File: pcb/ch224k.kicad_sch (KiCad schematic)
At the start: 3 parts, among them SW1 SW_Push_DPDT, U2 CH224K

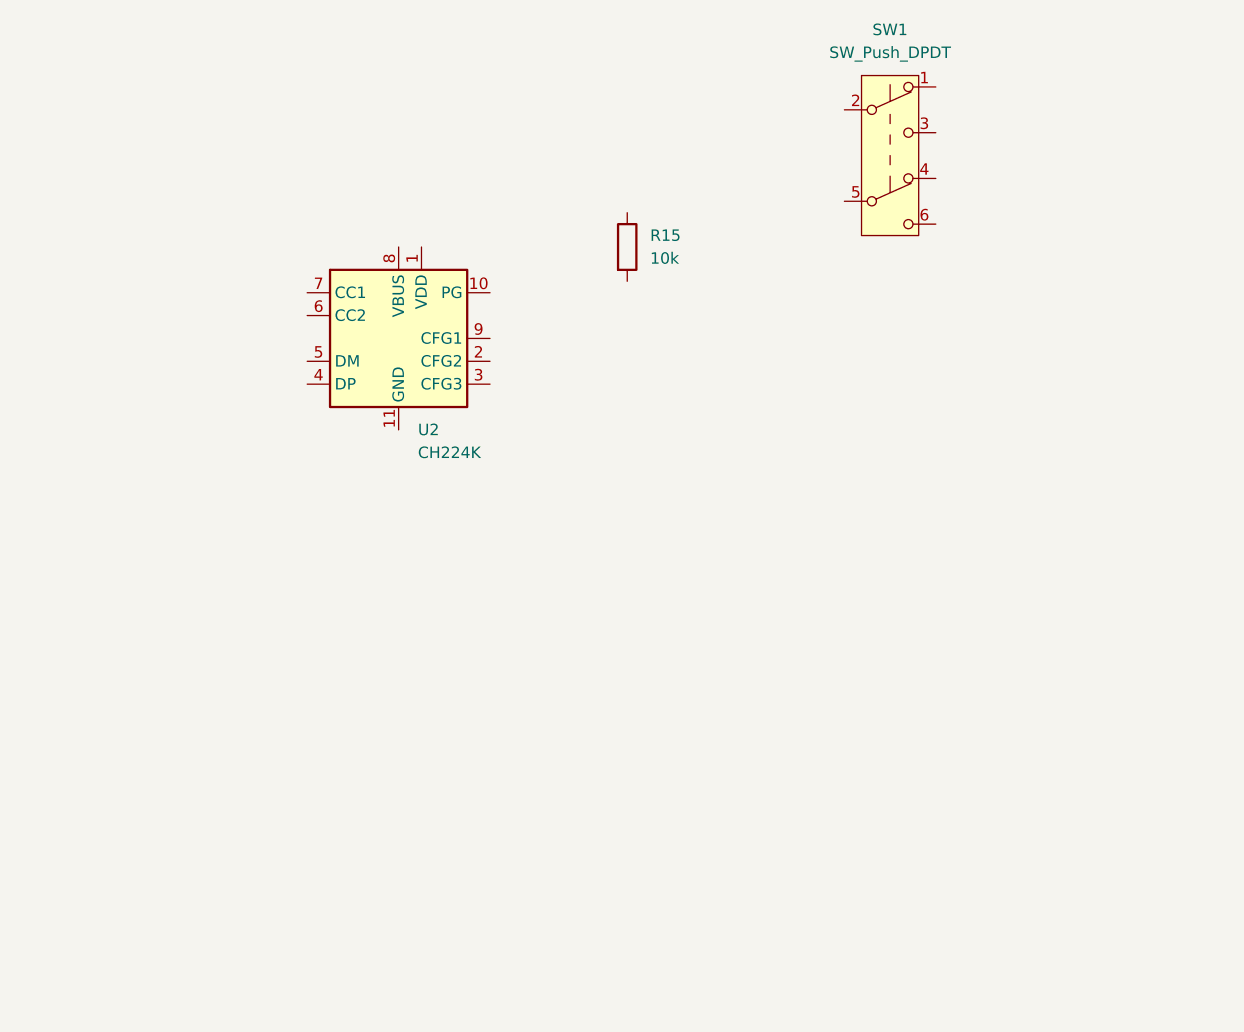
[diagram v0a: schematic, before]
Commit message: 提交信息
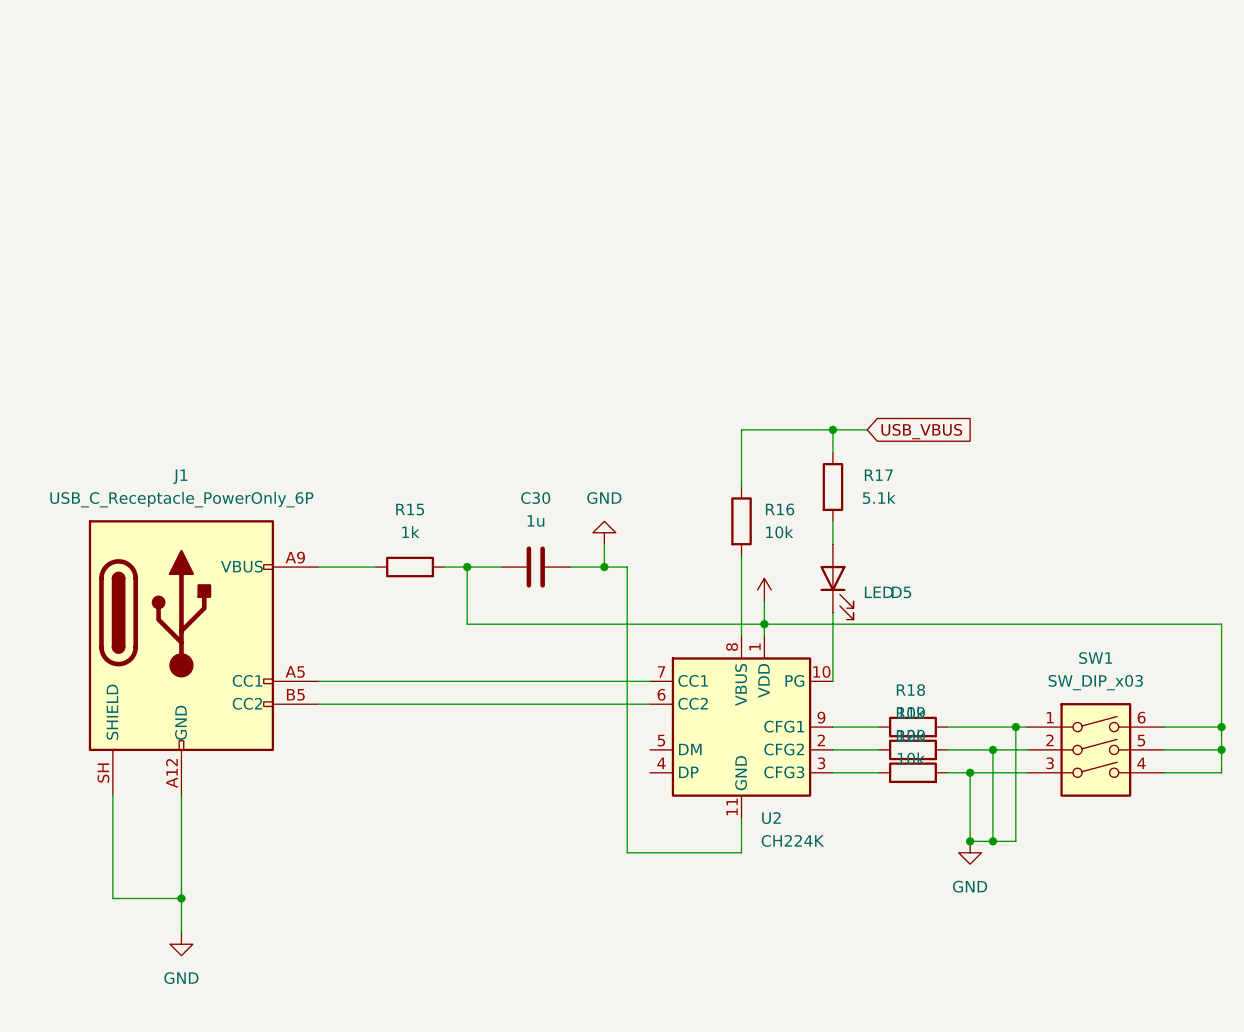
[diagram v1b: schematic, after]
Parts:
- removed SW1: SW_Push_DPDT, lcsc_pro:SW-SMD_6P-L9.1-W3.5-P2.50, symbol Switch:SW_Push_DPDT
- added C30: 1u, Capacitor_SMD:C_0805_2012Metric, symbol Device:C
- added D5: LED, LED_SMD:LED_0805_2012Metric, symbol Device:LED
- added J1: USB_C_Receptacle_PowerOnly_6P, Connector_USB:USB_C_Receptacle_GCT_USB4125-xx-x-0190_6P_TopMnt_Horizontal, symbol Connector:USB_C_Receptacle_PowerOnly_6P
- added R16, R18, R19, R20: 10k, Resistor_SMD:R_0805_2012Metric, symbol Device:R
- added R17: 5.1k, Resistor_SMD:R_0805_2012Metric, symbol Device:R
- added SW1: SW_DIP_x03, Button_Switch_SMD:SW_DIP_SPSTx03_Slide_6.7x9.18mm_W8.61mm_P2.54mm_LowProfile, symbol Switch:SW_DIP_x03
- R15: value 10k -> 1k; footprint Capacitor_SMD:C_1206_3216Metric -> Resistor_SMD:R_0805_2012Metric
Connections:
- net at R15.1: now also J1.A9 (VBUS), J1.B9 (VBUS)
- net VDD: now reaches R15.2
- net VDD: now also U2.1 (VDD), C30.1, SW1.4, SW1.5, SW1.6
- net at U2.10 (PG): now also D5.1 (K)
- net GND: now reaches U2.11 (GND)
- net GND: now also C30.2, J1.A12 (GND), J1.B12 (GND), J1.SH (SHIELD), R18.2, R19.2, R20.2, SW1.1, SW1.2, SW1.3
- net at U2.2 (CFG2): now also R19.1
- net at U2.3 (CFG3): now also R20.1
- net at U2.6 (CC2): now also J1.B5 (CC2)
- net at U2.7 (CC1): now also J1.A5 (CC1)
- net at U2.8 (VBUS): now also R16.2
- net at U2.9 (CFG1): now also R18.1
- new net: D5.2 (A), R17.2
- new net USB_VBUS: R16.1, R17.1

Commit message: 添加6p typec沉板
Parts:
- J1: footprint Connector_USB:USB_C_Receptacle_GCT_USB4125-xx-x-0190_6P_TopMnt_Horizontal -> lcsc_pro:USB-TYPE-C-SMD_TYPE-C
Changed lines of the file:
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@@
 			)
 		)
-		(property "Footprint" "Connector_USB:USB_C_Receptacle_GCT_USB4125-xx-x-0190_6P_TopMnt_Horizontal"
+		(property "Footprint" "lcsc_pro:USB-TYPE-C-SMD_TYPE-C"
 			(at 106.68 100.33 0)
 			(hide yes)

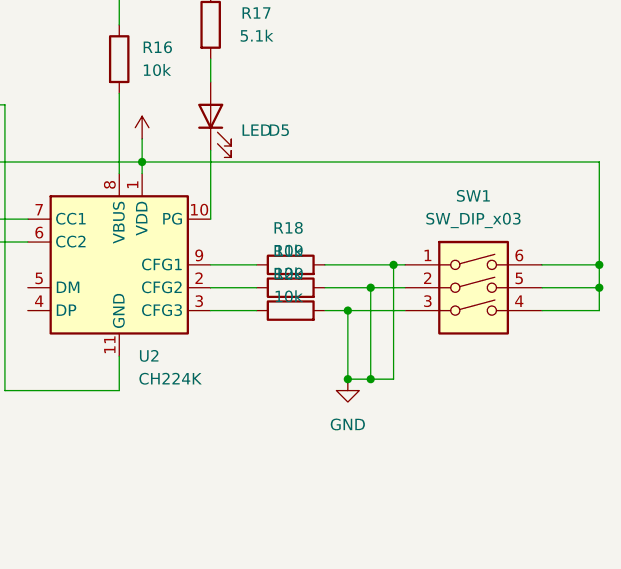
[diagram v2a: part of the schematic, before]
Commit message: 叫信息
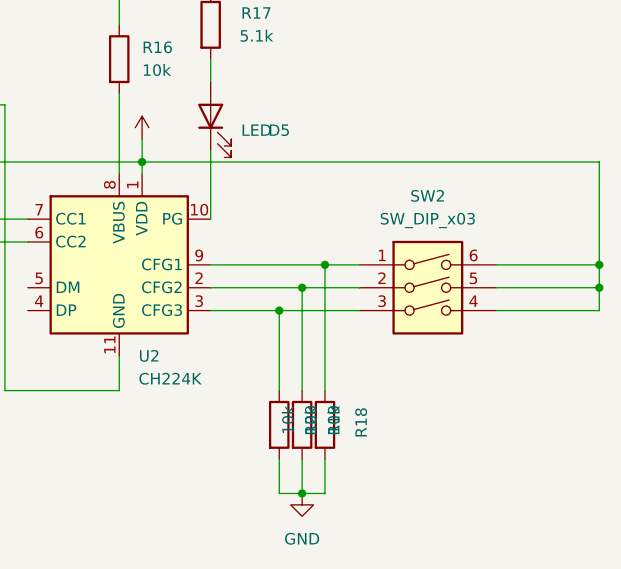
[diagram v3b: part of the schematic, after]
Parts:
- removed SW1: SW_DIP_x03, Button_Switch_SMD:SW_DIP_SPSTx03_Slide_6.7x9.18mm_W8.61mm_P2.54mm_LowProfile, symbol Switch:SW_DIP_x03
- added SW2: SW_DIP_x03, Button_Switch_SMD:SW_DIP_SPSTx03_Slide_6.7x9.18mm_W8.61mm_P2.54mm_LowProfile, symbol Switch:SW_DIP_x03
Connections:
- net VDD: now also SW2.4, SW2.5, SW2.6
- net at R18.1, U2.9 (CFG1): now also SW2.1
- net at R19.1, U2.2 (CFG2): now also SW2.2
- net at R20.1, U2.3 (CFG3): now also SW2.3
